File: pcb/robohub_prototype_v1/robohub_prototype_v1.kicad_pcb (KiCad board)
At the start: 10 copper layers, 102 parts, among them J21 Barrel_Jack_Switch_Pin3Ring, J51 USB_A, J52 USB_A, J71 USB_A, U1 ATSAMA5D27C, U21 LM3880, U22 TPS564242DRL, U23 TPS564242DRL, U24 TPS564242DRL, U25 TPS564242DRL, U26 TPS564242DRL, U27 TPS564242DRL, U31 W972GG6KB-25, U32 W972GG6KB-25, U41 KSZ8081RNB, U42 SI-60110-F, U61 molex_5025700893, U71 MCP2200-I-SO, X41 ECS-2520MV-xxx-xx

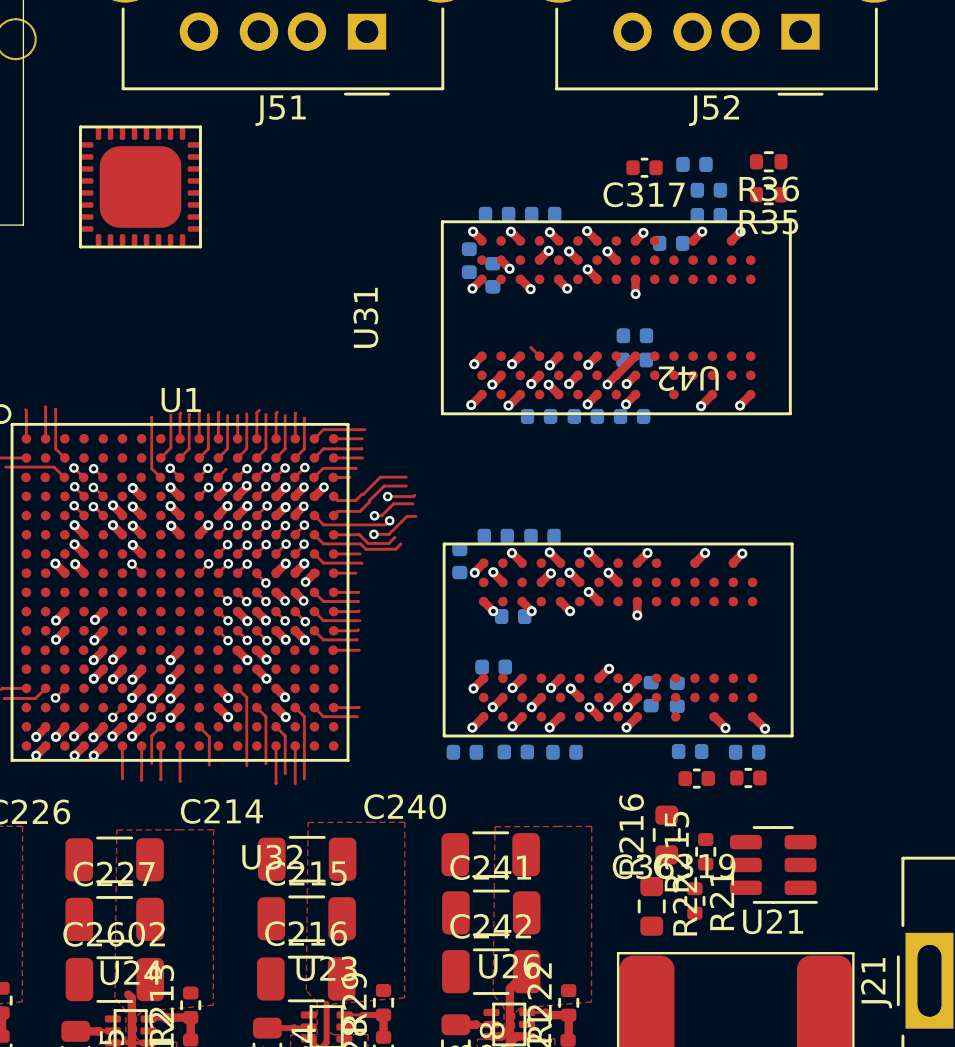
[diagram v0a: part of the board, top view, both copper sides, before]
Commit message: Moved some stuff around, tried a route
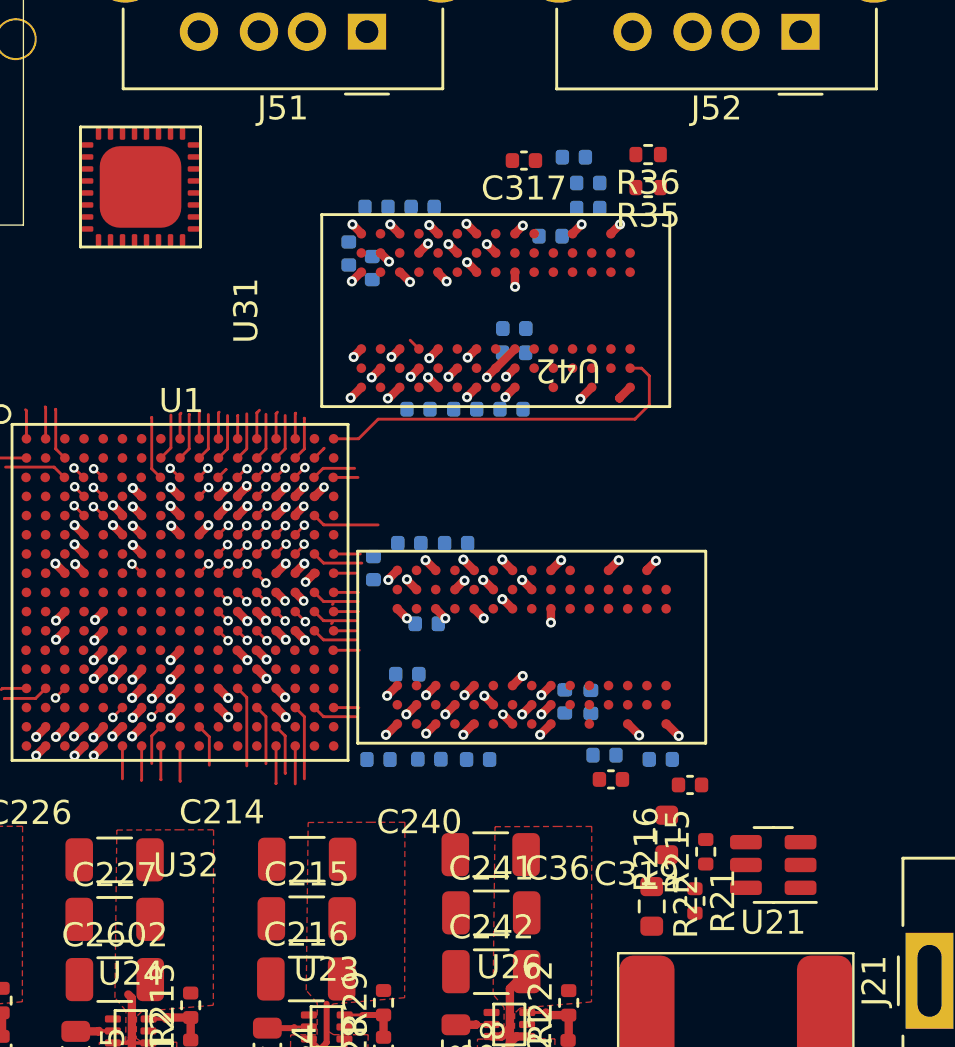
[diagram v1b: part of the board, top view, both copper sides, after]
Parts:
- moved C310 5.03 mm to (133.7, 87.1)
- moved C312 5.03 mm to (131.8, 87.1)
- moved C320 5.03 mm to (138.9, 78.7)
- moved C331 5.03 mm to (135.8, 83.7)
- moved C37 5.03 mm to (138.3, 76.6)
- moved C39 5.03 mm to (135.7, 87.1)
- moved R35 5.03 mm to (141.3, 77.8)
- moved R36 5.03 mm to (141.3, 76.5)
- moved U31 5.03 mm to (135.0, 83.0)
- moved C321 5.03 mm to (130.0, 78.7)
- moved C325 5.03 mm to (129.9, 81.2)
- moved C327 5.03 mm to (128.9, 80.6)
- moved C328 5.03 mm to (137.3, 79.9)
- moved C330 5.03 mm to (135.8, 84.7)
- moved C38 5.03 mm to (138.9, 77.7)
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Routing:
- net /DDR2_3/DDR_A12: track 1.19 -> 15.9 mm
- net /DDR2_3/DDR_A7: track 9.23 -> 0.90 mm, vias 2 -> 1
- net /DDR2_3/DDR_A13: track 8.91 -> 0.57 mm, vias 2 -> 1
- net /DDR2_3/DDR_A0: track 7.89 -> 0.58 mm, vias 2 -> 1
- net /DDR2_3/DDR_CKE: track 3.94 -> 0.00 mm
- net /DDR2_3/DDR_CLK+: track 3.57 -> 0.00 mm
- net /DDR2_3/DDR_CLK-: track 3.58 -> 0.15 mm
- net /DDR2_3/DDR_BA2: track 2.82 -> 0.01 mm
- net /DDR2_3/DDR_A11: track 2.25 -> 0.00 mm
- net /DDR2_3/DDR_A3: track 2.14 -> 0.67 mm
- net /DDR2_3/DDR_A2: track 1.21 -> 0.00 mm
- net Net-(U1E-DDR_RESETN): track 3.37 -> 2.81 mm, vias 1 -> 0
- net VCC_1_8_DDR: vias 39 -> 38
